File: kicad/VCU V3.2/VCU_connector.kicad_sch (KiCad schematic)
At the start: 2 parts

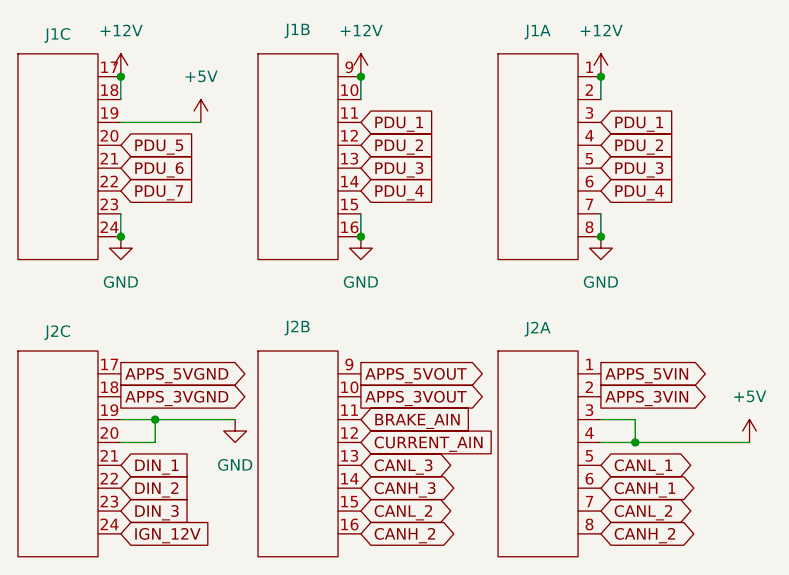
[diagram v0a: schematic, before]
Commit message: pudh
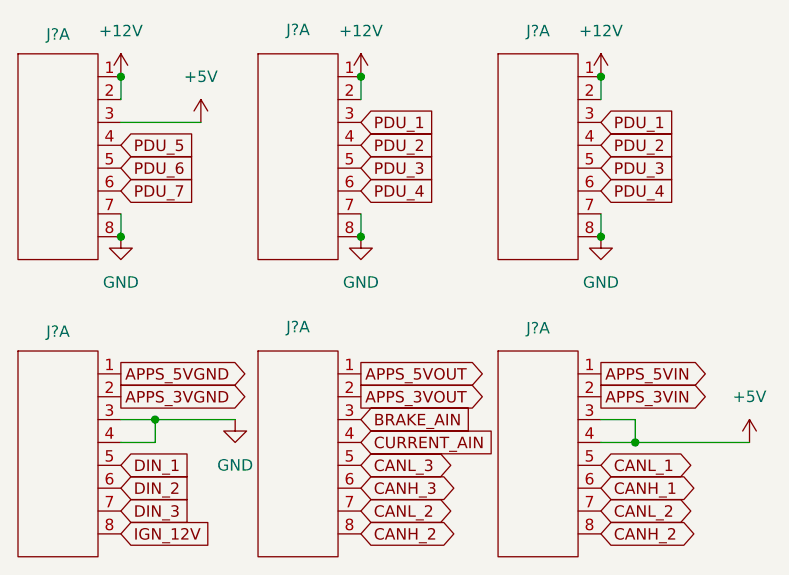
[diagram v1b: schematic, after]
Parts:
- renumbered J2 to J?, J1 to J?
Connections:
- net +12V: now also J?.1, J?.1, J?.2, J?.2; no longer J?.10, J?.17, J?.18, J?.9
- net +5V: now also J?.3; no longer J?.19
- net APPS_3VGND: now also J?.2; no longer J?.18
- net APPS_3VOUT: now also J?.2; no longer J?.10
- net APPS_5VGND: now also J?.1; no longer J?.17
- net APPS_5VOUT: now also J?.1; no longer J?.9
- net BRAKE_AIN: now also J?.3; no longer J?.11
- net CANH_2: now also J?.8; no longer J?.16
- net CANH_3: now also J?.6; no longer J?.14
- net CANL_2: now also J?.7; no longer J?.15
- net CANL_3: now also J?.5; no longer J?.13
- net CURRENT_AIN: now also J?.4; no longer J?.12
- net DIN_1: now also J?.5; no longer J?.21
- net DIN_2: now also J?.6; no longer J?.22
- net DIN_3: now also J?.7; no longer J?.23
- net GND: now also J?.3, J?.4, J?.7, J?.7, J?.8, J?.8; no longer J?.15, J?.16, J?.19, J?.20, J?.23, J?.24
- net IGN_12V: now also J?.8; no longer J?.24
- net PDU_1: now also J?.3; no longer J?.11
- net PDU_2: now also J?.4; no longer J?.12
- net PDU_3: now also J?.5; no longer J?.13
- net PDU_4: now also J?.6; no longer J?.14
- net PDU_5: now also J?.4; no longer J?.20
- net PDU_6: now also J?.5; no longer J?.21
- net PDU_7: now also J?.6; no longer J?.22
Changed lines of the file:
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@@
 		(dnp no)
 		(fields_autoplaced yes)
-		(property "Reference" "#PWR04"
+		(property "Reference" "#PWR?"
 			(at 90.17 76.2 0)
 			(effects
@@
 		(dnp no)
 		(fields_autoplaced yes)
-		(property "Reference" "#PWR015"
+		(property "Reference" "#PWR?"
 			(at 143.51 76.2 0)
 			(effects
@@
 		(dnp no)
 		(fields_autoplaced yes)
-		(property "Reference" "#PWR08"
+		(property "Reference" "#PWR?"
 			(at 99.06 81.28 0)
 			(effects
@@
 		(dnp no)
 		(fields_autoplaced yes)
-		(property "Reference" "#PWR010"
+		(property "Reference" "#PWR?"
 			(at 102.87 116.84 0)
 			(effects
@@
 		(lib_id "HD241:HD241")
 		(at 105.41 102.87 0)
-		(unit 2)
-		(exclude_from_sim no)
-		(in_bom yes)
-		(on_board yes)
-		(dnp no)
-		(fields_autoplaced yes)
-		(property "Reference" "J2"
+		(unit 1)
+		(exclude_from_sim no)
+		(in_bom yes)
+		(on_board yes)
+		(dnp no)
+		(fields_autoplaced yes)
+		(property "Reference" "J?"
 			(at 109.855 100.203 0)
 			(effects
@@
 		(dnp no)
 		(fields_autoplaced yes)
-		(property "Reference" "J2"
+		(property "Reference" "J?"
 			(at 136.525 100.33 0)
 			(effects
@@
 		(dnp no)
 		(fields_autoplaced yes)
-		(property "Reference" "#PWR05"
+		(property "Reference" "#PWR?"
 			(at 90.17 96.52 0)
 			(effects
@@
 		(lib_id "HD241:HD241")
 		(at 78.74 69.85 0)
-		(unit 3)
-		(exclude_from_sim no)
-		(in_bom yes)
-		(on_board yes)
-		(dnp no)
-		(fields_autoplaced yes)
-		(property "Reference" "J1"
+		(unit 1)
+		(exclude_from_sim no)
+		(in_bom yes)
+		(on_board yes)
+		(dnp no)
+		(fields_autoplaced yes)
+		(property "Reference" "J?"
 			(at 83.185 67.691 0)
 			(effects
@@
 		(dnp no)
 		(fields_autoplaced yes)
-		(property "Reference" "#PWR018"
+		(property "Reference" "#PWR?"
 			(at 160.02 116.84 0)
 			(effects
@@
 		(lib_id "HD241:HD241")
 		(at 105.41 69.85 0)
-		(unit 2)
-		(exclude_from_sim no)
-		(in_bom yes)
-		(on_board yes)
-		(dnp no)
-		(fields_autoplaced yes)
-		(property "Reference" "J1"
+		(unit 1)
+		(exclude_from_sim no)
+		(in_bom yes)
+		(on_board yes)
+		(dnp no)
+		(fields_autoplaced yes)
+		(property "Reference" "J?"
 			(at 109.855 67.183 0)
 			(effects
@@
 		(dnp no)
 		(fields_autoplaced yes)
-		(property "Reference" "J1"
+		(property "Reference" "J?"
 			(at 136.525 67.31 0)
 			(effects
@@
 		(dnp no)
 		(fields_autoplaced yes)
-		(property "Reference" "#PWR016"
+		(property "Reference" "#PWR?"
 			(at 143.51 96.52 0)
 			(effects
@@
 		(dnp no)
 		(fields_autoplaced yes)
-		(property "Reference" "#PWR013"
+		(property "Reference" "#PWR?"
 			(at 116.84 76.2 0)
 			(effects
@@
 		(lib_id "HD241:HD241")
 		(at 78.74 102.87 0)
-		(unit 3)
-		(exclude_from_sim no)
-		(in_bom yes)
-		(on_board yes)
-		(dnp no)
-		(fields_autoplaced yes)
-		(property "Reference" "J2"
+		(unit 1)
+		(exclude_from_sim no)
+		(in_bom yes)
+		(on_board yes)
+		(dnp no)
+		(fields_autoplaced yes)
+		(property "Reference" "J?"
 			(at 83.185 100.711 0)
 			(effects
@@
 		(dnp no)
 		(fields_autoplaced yes)
-		(property "Reference" "#PWR014"
+		(property "Reference" "#PWR?"
 			(at 116.84 96.52 0)
 			(effects
